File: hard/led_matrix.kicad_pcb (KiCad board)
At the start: 2 copper layers, 150 x 150 mm, 14 parts, among them J1 MicroXNJ

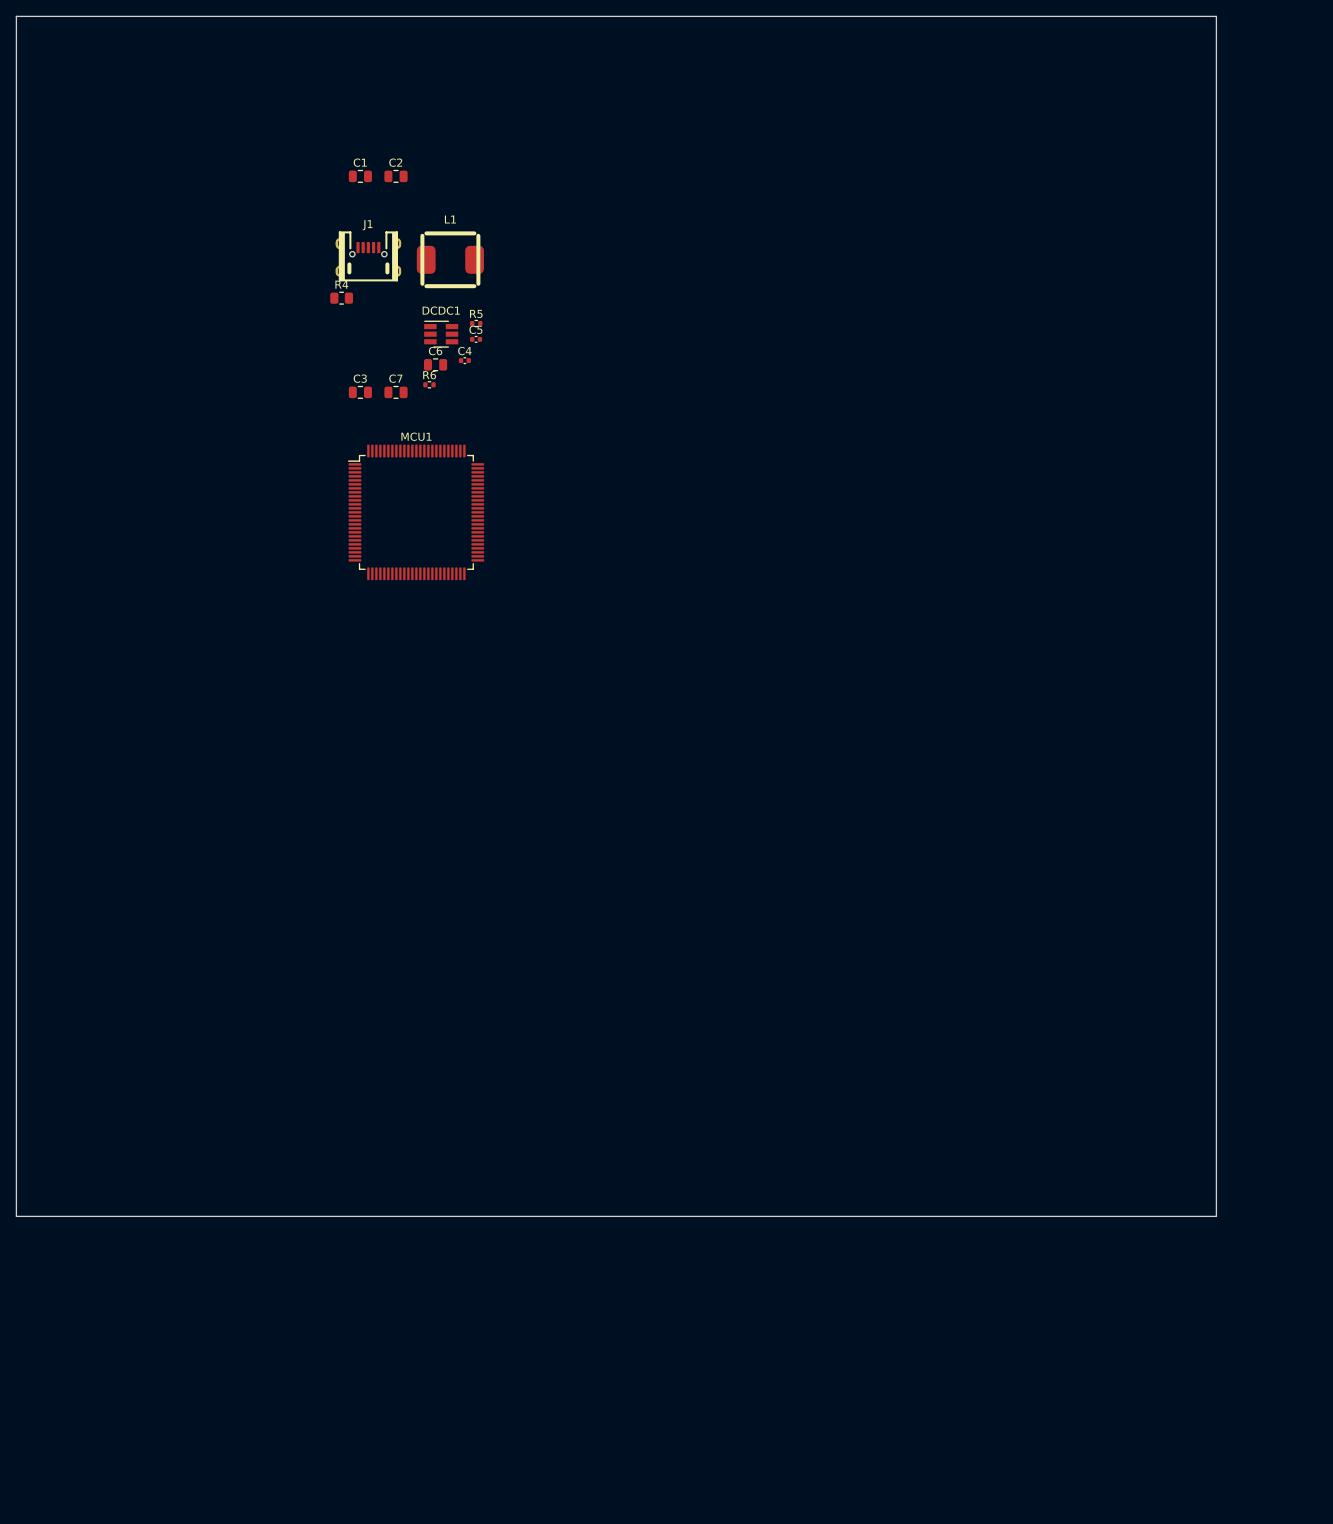
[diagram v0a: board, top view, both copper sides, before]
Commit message: RIIIIIIIIIIIIIBSSSSSS!!!!
Rib break
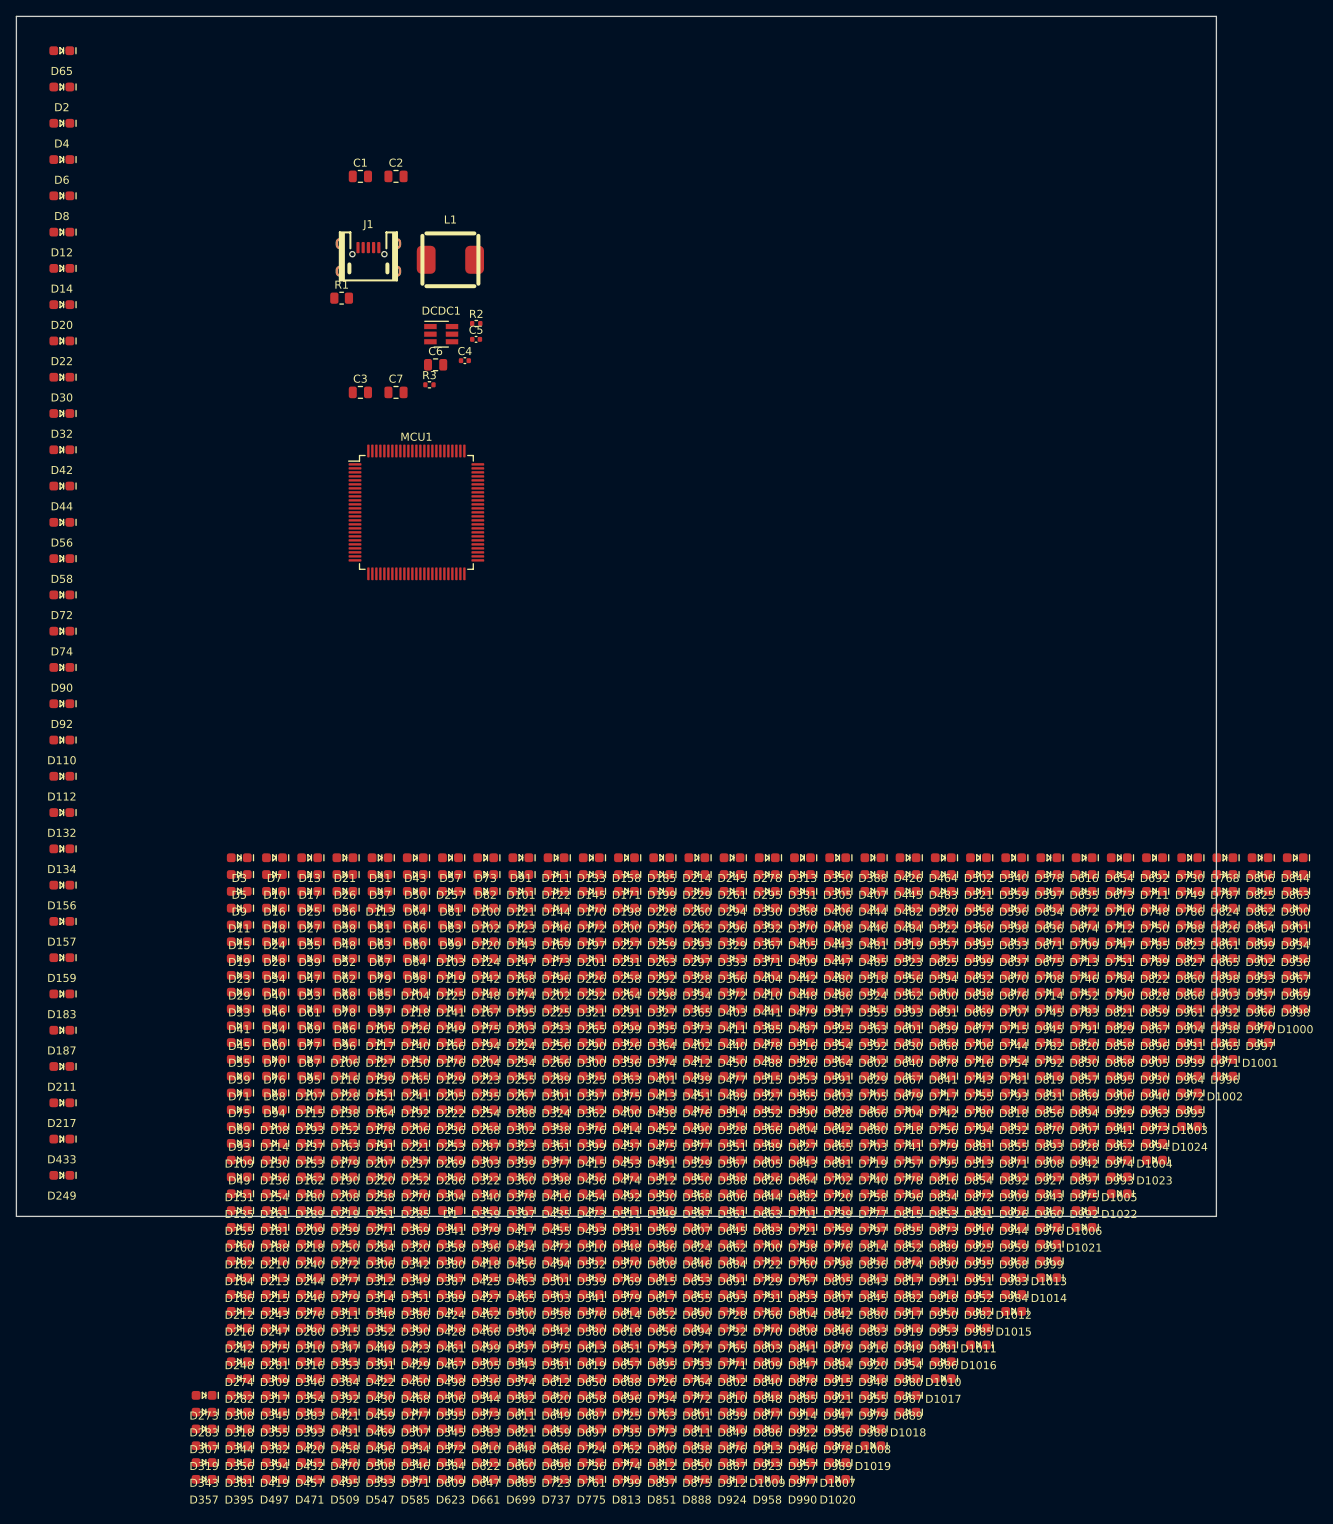
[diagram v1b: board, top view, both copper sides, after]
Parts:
- added D1: LTST-S270TBKT, led_matrix:LED_LiteOn_LTST-S270TBKT, F.Cu at (74.3, 177.2)
- added D10: LTST-S270TBKT, led_matrix:LED_LiteOn_LTST-S270TBKT, F.Cu at (52.3, 137.3)
- added D100: LTST-S270TBKT, led_matrix:LED_LiteOn_LTST-S270TBKT, F.Cu at (78.7, 139.4)
- added D1000: LTST-S270TBKT, led_matrix:LED_LiteOn_LTST-S270TBKT, F.Cu at (179.9, 154.1)
- added D1001: LTST-S270TBKT, led_matrix:LED_LiteOn_LTST-S270TBKT, F.Cu at (175.5, 158.3)
- added D1002: LTST-S270TBKT, led_matrix:LED_LiteOn_LTST-S270TBKT, F.Cu at (171.1, 162.5)
- added D1003: LTST-S270TBKT, led_matrix:LED_LiteOn_LTST-S270TBKT, F.Cu at (166.7, 166.7)
- added D1004: LTST-S270TBKT, led_matrix:LED_LiteOn_LTST-S270TBKT, F.Cu at (162.3, 170.9)
- added D1005: LTST-S270TBKT, led_matrix:LED_LiteOn_LTST-S270TBKT, F.Cu at (157.9, 175.1)
- added D1006: LTST-S270TBKT, led_matrix:LED_LiteOn_LTST-S270TBKT, F.Cu at (153.5, 179.3)
- added D1007: LTST-S270TBKT, led_matrix:LED_LiteOn_LTST-S270TBKT, F.Cu at (122.7, 210.8)
- added D1008: LTST-S270TBKT, led_matrix:LED_LiteOn_LTST-S270TBKT, F.Cu at (127.1, 206.6)
- added D1009: LTST-S270TBKT, led_matrix:LED_LiteOn_LTST-S270TBKT, F.Cu at (113.9, 210.8)
- added D101: LTST-S270TBKT, led_matrix:LED_LiteOn_LTST-S270TBKT, F.Cu at (83.1, 137.3)
- added D1010: LTST-S270TBKT, led_matrix:LED_LiteOn_LTST-S270TBKT, F.Cu at (135.9, 198.2)
- added D1011: LTST-S270TBKT, led_matrix:LED_LiteOn_LTST-S270TBKT, F.Cu at (140.3, 194.0)
- added D1012: LTST-S270TBKT, led_matrix:LED_LiteOn_LTST-S270TBKT, F.Cu at (144.7, 189.8)
- added D1013: LTST-S270TBKT, led_matrix:LED_LiteOn_LTST-S270TBKT, F.Cu at (149.1, 185.6)
- added D1014: LTST-S270TBKT, led_matrix:LED_LiteOn_LTST-S270TBKT, F.Cu at (149.1, 187.7)
- added D1015: LTST-S270TBKT, led_matrix:LED_LiteOn_LTST-S270TBKT, F.Cu at (144.7, 191.9)
- added D1016: LTST-S270TBKT, led_matrix:LED_LiteOn_LTST-S270TBKT, F.Cu at (140.3, 196.1)
- added D1017: LTST-S270TBKT, led_matrix:LED_LiteOn_LTST-S270TBKT, F.Cu at (135.9, 200.3)
- added D1018: LTST-S270TBKT, led_matrix:LED_LiteOn_LTST-S270TBKT, F.Cu at (131.5, 204.5)
- added D1019: LTST-S270TBKT, led_matrix:LED_LiteOn_LTST-S270TBKT, F.Cu at (127.1, 208.7)
- added D102: LTST-S270TBKT, led_matrix:LED_LiteOn_LTST-S270TBKT, F.Cu at (78.7, 141.5)
- added D1020: LTST-S270TBKT, led_matrix:LED_LiteOn_LTST-S270TBKT, F.Cu at (122.7, 212.9)
- added D1021: LTST-S270TBKT, led_matrix:LED_LiteOn_LTST-S270TBKT, F.Cu at (153.5, 181.4)
- added D1022: LTST-S270TBKT, led_matrix:LED_LiteOn_LTST-S270TBKT, F.Cu at (157.9, 177.2)
- added D1023: LTST-S270TBKT, led_matrix:LED_LiteOn_LTST-S270TBKT, F.Cu at (162.3, 173.0)
- added D1024: LTST-S270TBKT, led_matrix:LED_LiteOn_LTST-S270TBKT, F.Cu at (166.7, 168.8)
- added D103: LTST-S270TBKT, led_matrix:LED_LiteOn_LTST-S270TBKT, F.Cu at (74.3, 145.7)
- added D104: LTST-S270TBKT, led_matrix:LED_LiteOn_LTST-S270TBKT, F.Cu at (69.9, 149.9)
- added D105: LTST-S270TBKT, led_matrix:LED_LiteOn_LTST-S270TBKT, F.Cu at (65.5, 154.1)
- added D106: LTST-S270TBKT, led_matrix:LED_LiteOn_LTST-S270TBKT, F.Cu at (61.1, 158.3)
- added D107: LTST-S270TBKT, led_matrix:LED_LiteOn_LTST-S270TBKT, F.Cu at (56.7, 162.5)
- added D108: LTST-S270TBKT, led_matrix:LED_LiteOn_LTST-S270TBKT, F.Cu at (52.3, 166.7)
- added D109: LTST-S270TBKT, led_matrix:LED_LiteOn_LTST-S270TBKT, F.Cu at (47.9, 170.9)
- added D11: LTST-S270TBKT, led_matrix:LED_LiteOn_LTST-S270TBKT, F.Cu at (47.9, 141.5)
- added D110: LTST-S270TBKT, led_matrix:LED_LiteOn_LTST-S270TBKT, F.Cu at (25.7, 120.5)
- added D111: LTST-S270TBKT, led_matrix:LED_LiteOn_LTST-S270TBKT, F.Cu at (87.5, 135.2)
- added D112: LTST-S270TBKT, led_matrix:LED_LiteOn_LTST-S270TBKT, F.Cu at (25.7, 125.0)
- added D113: LTST-S270TBKT, led_matrix:LED_LiteOn_LTST-S270TBKT, F.Cu at (65.5, 139.4)
- added D114: LTST-S270TBKT, led_matrix:LED_LiteOn_LTST-S270TBKT, F.Cu at (52.3, 168.8)
- added D115: LTST-S270TBKT, led_matrix:LED_LiteOn_LTST-S270TBKT, F.Cu at (56.7, 164.6)
- added D116: LTST-S270TBKT, led_matrix:LED_LiteOn_LTST-S270TBKT, F.Cu at (61.1, 160.4)
- added D117: LTST-S270TBKT, led_matrix:LED_LiteOn_LTST-S270TBKT, F.Cu at (65.5, 156.2)
- added D118: LTST-S270TBKT, led_matrix:LED_LiteOn_LTST-S270TBKT, F.Cu at (69.9, 152.0)
- added D119: LTST-S270TBKT, led_matrix:LED_LiteOn_LTST-S270TBKT, F.Cu at (74.3, 147.8)
- added D12: LTST-S270TBKT, led_matrix:LED_LiteOn_LTST-S270TBKT, F.Cu at (25.7, 57.0)
- added D120: LTST-S270TBKT, led_matrix:LED_LiteOn_LTST-S270TBKT, F.Cu at (78.7, 143.6)
- added D121: LTST-S270TBKT, led_matrix:LED_LiteOn_LTST-S270TBKT, F.Cu at (83.1, 139.4)
- added D122: LTST-S270TBKT, led_matrix:LED_LiteOn_LTST-S270TBKT, F.Cu at (87.5, 137.3)
- added D123: LTST-S270TBKT, led_matrix:LED_LiteOn_LTST-S270TBKT, F.Cu at (83.1, 141.5)
- added D124: LTST-S270TBKT, led_matrix:LED_LiteOn_LTST-S270TBKT, F.Cu at (78.7, 145.7)
- added D125: LTST-S270TBKT, led_matrix:LED_LiteOn_LTST-S270TBKT, F.Cu at (74.3, 149.9)
- added D126: LTST-S270TBKT, led_matrix:LED_LiteOn_LTST-S270TBKT, F.Cu at (69.9, 154.1)
- added D127: LTST-S270TBKT, led_matrix:LED_LiteOn_LTST-S270TBKT, F.Cu at (65.5, 158.3)
- added D128: LTST-S270TBKT, led_matrix:LED_LiteOn_LTST-S270TBKT, F.Cu at (61.1, 162.5)
- added D129: LTST-S270TBKT, led_matrix:LED_LiteOn_LTST-S270TBKT, F.Cu at (74.3, 160.4)
- added D13: LTST-S270TBKT, led_matrix:LED_LiteOn_LTST-S270TBKT, F.Cu at (56.7, 135.2)
- added D130: LTST-S270TBKT, led_matrix:LED_LiteOn_LTST-S270TBKT, F.Cu at (52.3, 170.9)
- added D131: LTST-S270TBKT, led_matrix:LED_LiteOn_LTST-S270TBKT, F.Cu at (47.9, 175.1)
- added D132: LTST-S270TBKT, led_matrix:LED_LiteOn_LTST-S270TBKT, F.Cu at (25.7, 129.5)
- added D133: LTST-S270TBKT, led_matrix:LED_LiteOn_LTST-S270TBKT, F.Cu at (91.9, 135.2)
- added D134: LTST-S270TBKT, led_matrix:LED_LiteOn_LTST-S270TBKT, F.Cu at (25.7, 134.1)
- added D135: LTST-S270TBKT, led_matrix:LED_LiteOn_LTST-S270TBKT, F.Cu at (47.9, 177.2)
- added D136: LTST-S270TBKT, led_matrix:LED_LiteOn_LTST-S270TBKT, F.Cu at (52.3, 173.0)
- added D137: LTST-S270TBKT, led_matrix:LED_LiteOn_LTST-S270TBKT, F.Cu at (56.7, 168.8)
- added D138: LTST-S270TBKT, led_matrix:LED_LiteOn_LTST-S270TBKT, F.Cu at (61.1, 164.6)
- added D139: LTST-S270TBKT, led_matrix:LED_LiteOn_LTST-S270TBKT, F.Cu at (65.5, 160.4)
- added D14: LTST-S270TBKT, led_matrix:LED_LiteOn_LTST-S270TBKT, F.Cu at (25.7, 61.5)
- added D140: LTST-S270TBKT, led_matrix:LED_LiteOn_LTST-S270TBKT, F.Cu at (69.9, 156.2)
- added D141: LTST-S270TBKT, led_matrix:LED_LiteOn_LTST-S270TBKT, F.Cu at (74.3, 152.0)
- added D142: LTST-S270TBKT, led_matrix:LED_LiteOn_LTST-S270TBKT, F.Cu at (78.7, 147.8)
- added D143: LTST-S270TBKT, led_matrix:LED_LiteOn_LTST-S270TBKT, F.Cu at (83.1, 143.6)
- added D144: LTST-S270TBKT, led_matrix:LED_LiteOn_LTST-S270TBKT, F.Cu at (87.5, 139.4)
- added D145: LTST-S270TBKT, led_matrix:LED_LiteOn_LTST-S270TBKT, F.Cu at (91.9, 137.3)
- added D146: LTST-S270TBKT, led_matrix:LED_LiteOn_LTST-S270TBKT, F.Cu at (87.5, 141.5)
- added D147: LTST-S270TBKT, led_matrix:LED_LiteOn_LTST-S270TBKT, F.Cu at (83.1, 145.7)
- added D148: LTST-S270TBKT, led_matrix:LED_LiteOn_LTST-S270TBKT, F.Cu at (78.7, 149.9)
- added D149: LTST-S270TBKT, led_matrix:LED_LiteOn_LTST-S270TBKT, F.Cu at (74.3, 154.1)
- added D15: LTST-S270TBKT, led_matrix:LED_LiteOn_LTST-S270TBKT, F.Cu at (47.9, 143.6)
- added D150: LTST-S270TBKT, led_matrix:LED_LiteOn_LTST-S270TBKT, F.Cu at (69.9, 158.3)
- added D151: LTST-S270TBKT, led_matrix:LED_LiteOn_LTST-S270TBKT, F.Cu at (65.5, 162.5)
- added D152: LTST-S270TBKT, led_matrix:LED_LiteOn_LTST-S270TBKT, F.Cu at (61.1, 166.7)
- added D153: LTST-S270TBKT, led_matrix:LED_LiteOn_LTST-S270TBKT, F.Cu at (56.7, 170.9)
- added D154: LTST-S270TBKT, led_matrix:LED_LiteOn_LTST-S270TBKT, F.Cu at (52.3, 175.1)
- added D155: LTST-S270TBKT, led_matrix:LED_LiteOn_LTST-S270TBKT, F.Cu at (47.9, 179.3)
- added D156: LTST-S270TBKT, led_matrix:LED_LiteOn_LTST-S270TBKT, F.Cu at (25.7, 138.6)
- added D157: LTST-S270TBKT, led_matrix:LED_LiteOn_LTST-S270TBKT, F.Cu at (25.7, 143.1)
- added D158: LTST-S270TBKT, led_matrix:LED_LiteOn_LTST-S270TBKT, F.Cu at (96.3, 135.2)
- added D159: LTST-S270TBKT, led_matrix:LED_LiteOn_LTST-S270TBKT, F.Cu at (25.7, 147.7)
- added D16: LTST-S270TBKT, led_matrix:LED_LiteOn_LTST-S270TBKT, F.Cu at (52.3, 139.4)
- added D160: LTST-S270TBKT, led_matrix:LED_LiteOn_LTST-S270TBKT, F.Cu at (47.9, 181.4)
- added D161: LTST-S270TBKT, led_matrix:LED_LiteOn_LTST-S270TBKT, F.Cu at (52.3, 177.2)
- added D162: LTST-S270TBKT, led_matrix:LED_LiteOn_LTST-S270TBKT, F.Cu at (56.7, 173.0)
- added D163: LTST-S270TBKT, led_matrix:LED_LiteOn_LTST-S270TBKT, F.Cu at (61.1, 168.8)
- added D164: LTST-S270TBKT, led_matrix:LED_LiteOn_LTST-S270TBKT, F.Cu at (65.5, 164.6)
- added D165: LTST-S270TBKT, led_matrix:LED_LiteOn_LTST-S270TBKT, F.Cu at (69.9, 160.4)
- added D166: LTST-S270TBKT, led_matrix:LED_LiteOn_LTST-S270TBKT, F.Cu at (74.3, 156.2)
- added D167: LTST-S270TBKT, led_matrix:LED_LiteOn_LTST-S270TBKT, F.Cu at (78.7, 152.0)
- added D168: LTST-S270TBKT, led_matrix:LED_LiteOn_LTST-S270TBKT, F.Cu at (83.1, 147.8)
- added D169: LTST-S270TBKT, led_matrix:LED_LiteOn_LTST-S270TBKT, F.Cu at (87.5, 143.6)
- added D17: LTST-S270TBKT, led_matrix:LED_LiteOn_LTST-S270TBKT, F.Cu at (56.7, 137.3)
- added D170: LTST-S270TBKT, led_matrix:LED_LiteOn_LTST-S270TBKT, F.Cu at (91.9, 139.4)
- added D171: LTST-S270TBKT, led_matrix:LED_LiteOn_LTST-S270TBKT, F.Cu at (96.3, 137.3)
- added D172: LTST-S270TBKT, led_matrix:LED_LiteOn_LTST-S270TBKT, F.Cu at (91.9, 141.5)
- added D173: LTST-S270TBKT, led_matrix:LED_LiteOn_LTST-S270TBKT, F.Cu at (87.5, 145.7)
- added D174: LTST-S270TBKT, led_matrix:LED_LiteOn_LTST-S270TBKT, F.Cu at (83.1, 149.9)
- added D175: LTST-S270TBKT, led_matrix:LED_LiteOn_LTST-S270TBKT, F.Cu at (78.7, 154.1)
- added D176: LTST-S270TBKT, led_matrix:LED_LiteOn_LTST-S270TBKT, F.Cu at (74.3, 158.3)
- added D177: LTST-S270TBKT, led_matrix:LED_LiteOn_LTST-S270TBKT, F.Cu at (69.9, 202.4)
- added D178: LTST-S270TBKT, led_matrix:LED_LiteOn_LTST-S270TBKT, F.Cu at (65.5, 166.7)
- added D179: LTST-S270TBKT, led_matrix:LED_LiteOn_LTST-S270TBKT, F.Cu at (61.1, 170.9)
- added D18: LTST-S270TBKT, led_matrix:LED_LiteOn_LTST-S270TBKT, F.Cu at (52.3, 141.5)
- added D180: LTST-S270TBKT, led_matrix:LED_LiteOn_LTST-S270TBKT, F.Cu at (56.7, 175.1)
- added D181: LTST-S270TBKT, led_matrix:LED_LiteOn_LTST-S270TBKT, F.Cu at (52.3, 179.3)
- added D182: LTST-S270TBKT, led_matrix:LED_LiteOn_LTST-S270TBKT, F.Cu at (47.9, 183.5)
- added D183: LTST-S270TBKT, led_matrix:LED_LiteOn_LTST-S270TBKT, F.Cu at (25.7, 152.2)
- added D184: LTST-S270TBKT, led_matrix:LED_LiteOn_LTST-S270TBKT, F.Cu at (47.9, 185.6)
- added D185: LTST-S270TBKT, led_matrix:LED_LiteOn_LTST-S270TBKT, F.Cu at (100.7, 135.2)
- added D186: LTST-S270TBKT, led_matrix:LED_LiteOn_LTST-S270TBKT, F.Cu at (47.9, 187.7)
- added D187: LTST-S270TBKT, led_matrix:LED_LiteOn_LTST-S270TBKT, F.Cu at (25.7, 156.7)
- added D188: LTST-S270TBKT, led_matrix:LED_LiteOn_LTST-S270TBKT, F.Cu at (52.3, 181.4)
- added D189: LTST-S270TBKT, led_matrix:LED_LiteOn_LTST-S270TBKT, F.Cu at (56.7, 177.2)
- added D19: LTST-S270TBKT, led_matrix:LED_LiteOn_LTST-S270TBKT, F.Cu at (47.9, 145.7)
- added D190: LTST-S270TBKT, led_matrix:LED_LiteOn_LTST-S270TBKT, F.Cu at (61.1, 173.0)
- added D191: LTST-S270TBKT, led_matrix:LED_LiteOn_LTST-S270TBKT, F.Cu at (65.5, 168.8)
- added D192: LTST-S270TBKT, led_matrix:LED_LiteOn_LTST-S270TBKT, F.Cu at (69.9, 164.6)
- added D193: LTST-S270TBKT, led_matrix:LED_LiteOn_LTST-S270TBKT, F.Cu at (56.7, 166.7)
- added D194: LTST-S270TBKT, led_matrix:LED_LiteOn_LTST-S270TBKT, F.Cu at (78.7, 156.2)
- added D195: LTST-S270TBKT, led_matrix:LED_LiteOn_LTST-S270TBKT, F.Cu at (83.1, 152.0)
- added D196: LTST-S270TBKT, led_matrix:LED_LiteOn_LTST-S270TBKT, F.Cu at (87.5, 147.8)
- added D197: LTST-S270TBKT, led_matrix:LED_LiteOn_LTST-S270TBKT, F.Cu at (91.9, 143.6)
- added D198: LTST-S270TBKT, led_matrix:LED_LiteOn_LTST-S270TBKT, F.Cu at (96.3, 139.4)
- added D199: LTST-S270TBKT, led_matrix:LED_LiteOn_LTST-S270TBKT, F.Cu at (100.7, 137.3)
- added D2: LTST-S270TBKT, led_matrix:LED_LiteOn_LTST-S270TBKT, F.Cu at (25.7, 38.8)
- added D20: LTST-S270TBKT, led_matrix:LED_LiteOn_LTST-S270TBKT, F.Cu at (25.7, 66.0)
- added D200: LTST-S270TBKT, led_matrix:LED_LiteOn_LTST-S270TBKT, F.Cu at (96.3, 141.5)
- added D201: LTST-S270TBKT, led_matrix:LED_LiteOn_LTST-S270TBKT, F.Cu at (91.9, 145.7)
- added D202: LTST-S270TBKT, led_matrix:LED_LiteOn_LTST-S270TBKT, F.Cu at (87.5, 149.9)
- added D203: LTST-S270TBKT, led_matrix:LED_LiteOn_LTST-S270TBKT, F.Cu at (83.1, 154.1)
- added D204: LTST-S270TBKT, led_matrix:LED_LiteOn_LTST-S270TBKT, F.Cu at (78.7, 158.3)
- added D205: LTST-S270TBKT, led_matrix:LED_LiteOn_LTST-S270TBKT, F.Cu at (74.3, 162.5)
- added D206: LTST-S270TBKT, led_matrix:LED_LiteOn_LTST-S270TBKT, F.Cu at (69.9, 166.7)
- added D207: LTST-S270TBKT, led_matrix:LED_LiteOn_LTST-S270TBKT, F.Cu at (65.5, 170.9)
- added D208: LTST-S270TBKT, led_matrix:LED_LiteOn_LTST-S270TBKT, F.Cu at (61.1, 175.1)
- added D209: LTST-S270TBKT, led_matrix:LED_LiteOn_LTST-S270TBKT, F.Cu at (56.7, 179.3)
- added D21: LTST-S270TBKT, led_matrix:LED_LiteOn_LTST-S270TBKT, F.Cu at (61.1, 135.2)
- added D210: LTST-S270TBKT, led_matrix:LED_LiteOn_LTST-S270TBKT, F.Cu at (52.3, 183.5)
- added D211: LTST-S270TBKT, led_matrix:LED_LiteOn_LTST-S270TBKT, F.Cu at (25.7, 161.3)
- added D212: LTST-S270TBKT, led_matrix:LED_LiteOn_LTST-S270TBKT, F.Cu at (47.9, 189.8)
- added D213: LTST-S270TBKT, led_matrix:LED_LiteOn_LTST-S270TBKT, F.Cu at (52.3, 185.6)
- added D214: LTST-S270TBKT, led_matrix:LED_LiteOn_LTST-S270TBKT, F.Cu at (105.1, 135.2)
- added D215: LTST-S270TBKT, led_matrix:LED_LiteOn_LTST-S270TBKT, F.Cu at (52.3, 187.7)
- added D216: LTST-S270TBKT, led_matrix:LED_LiteOn_LTST-S270TBKT, F.Cu at (47.9, 191.9)
- added D217: LTST-S270TBKT, led_matrix:LED_LiteOn_LTST-S270TBKT, F.Cu at (25.7, 165.8)
- added D218: LTST-S270TBKT, led_matrix:LED_LiteOn_LTST-S270TBKT, F.Cu at (56.7, 181.4)
- added D219: LTST-S270TBKT, led_matrix:LED_LiteOn_LTST-S270TBKT, F.Cu at (61.1, 177.2)
- added D22: LTST-S270TBKT, led_matrix:LED_LiteOn_LTST-S270TBKT, F.Cu at (25.7, 70.6)
- added D220: LTST-S270TBKT, led_matrix:LED_LiteOn_LTST-S270TBKT, F.Cu at (65.5, 173.0)
- added D221: LTST-S270TBKT, led_matrix:LED_LiteOn_LTST-S270TBKT, F.Cu at (69.9, 168.8)
- added D222: LTST-S270TBKT, led_matrix:LED_LiteOn_LTST-S270TBKT, F.Cu at (74.3, 164.6)
- added D223: LTST-S270TBKT, led_matrix:LED_LiteOn_LTST-S270TBKT, F.Cu at (78.7, 160.4)
- added D224: LTST-S270TBKT, led_matrix:LED_LiteOn_LTST-S270TBKT, F.Cu at (83.1, 156.2)
- added D225: LTST-S270TBKT, led_matrix:LED_LiteOn_LTST-S270TBKT, F.Cu at (87.5, 152.0)
- added D226: LTST-S270TBKT, led_matrix:LED_LiteOn_LTST-S270TBKT, F.Cu at (91.9, 147.8)
- added D227: LTST-S270TBKT, led_matrix:LED_LiteOn_LTST-S270TBKT, F.Cu at (96.3, 143.6)
- added D228: LTST-S270TBKT, led_matrix:LED_LiteOn_LTST-S270TBKT, F.Cu at (100.7, 139.4)
- added D229: LTST-S270TBKT, led_matrix:LED_LiteOn_LTST-S270TBKT, F.Cu at (105.1, 137.3)
- added D23: LTST-S270TBKT, led_matrix:LED_LiteOn_LTST-S270TBKT, F.Cu at (47.9, 147.8)
- added D230: LTST-S270TBKT, led_matrix:LED_LiteOn_LTST-S270TBKT, F.Cu at (100.7, 141.5)
- added D231: LTST-S270TBKT, led_matrix:LED_LiteOn_LTST-S270TBKT, F.Cu at (96.3, 145.7)
- added D232: LTST-S270TBKT, led_matrix:LED_LiteOn_LTST-S270TBKT, F.Cu at (91.9, 149.9)
- added D233: LTST-S270TBKT, led_matrix:LED_LiteOn_LTST-S270TBKT, F.Cu at (87.5, 154.1)
- added D234: LTST-S270TBKT, led_matrix:LED_LiteOn_LTST-S270TBKT, F.Cu at (83.1, 158.3)
- added D235: LTST-S270TBKT, led_matrix:LED_LiteOn_LTST-S270TBKT, F.Cu at (78.7, 162.5)
- added D236: LTST-S270TBKT, led_matrix:LED_LiteOn_LTST-S270TBKT, F.Cu at (74.3, 166.7)
- added D237: LTST-S270TBKT, led_matrix:LED_LiteOn_LTST-S270TBKT, F.Cu at (69.9, 170.9)
- added D238: LTST-S270TBKT, led_matrix:LED_LiteOn_LTST-S270TBKT, F.Cu at (65.5, 175.1)
- added D239: LTST-S270TBKT, led_matrix:LED_LiteOn_LTST-S270TBKT, F.Cu at (61.1, 179.3)
- added D24: LTST-S270TBKT, led_matrix:LED_LiteOn_LTST-S270TBKT, F.Cu at (52.3, 143.6)
- added D240: LTST-S270TBKT, led_matrix:LED_LiteOn_LTST-S270TBKT, F.Cu at (56.7, 183.5)
- added D241: LTST-S270TBKT, led_matrix:LED_LiteOn_LTST-S270TBKT, F.Cu at (69.9, 162.5)
- added D242: LTST-S270TBKT, led_matrix:LED_LiteOn_LTST-S270TBKT, F.Cu at (47.9, 194.0)
- added D243: LTST-S270TBKT, led_matrix:LED_LiteOn_LTST-S270TBKT, F.Cu at (52.3, 189.8)
- added D244: LTST-S270TBKT, led_matrix:LED_LiteOn_LTST-S270TBKT, F.Cu at (56.7, 185.6)
- added D245: LTST-S270TBKT, led_matrix:LED_LiteOn_LTST-S270TBKT, F.Cu at (109.5, 135.2)
- added D246: LTST-S270TBKT, led_matrix:LED_LiteOn_LTST-S270TBKT, F.Cu at (56.7, 187.7)
- added D247: LTST-S270TBKT, led_matrix:LED_LiteOn_LTST-S270TBKT, F.Cu at (52.3, 191.9)
- added D248: LTST-S270TBKT, led_matrix:LED_LiteOn_LTST-S270TBKT, F.Cu at (47.9, 196.1)
- added D249: LTST-S270TBKT, led_matrix:LED_LiteOn_LTST-S270TBKT, F.Cu at (25.7, 174.9)
- added D25: LTST-S270TBKT, led_matrix:LED_LiteOn_LTST-S270TBKT, F.Cu at (56.7, 139.4)
- added D250: LTST-S270TBKT, led_matrix:LED_LiteOn_LTST-S270TBKT, F.Cu at (61.1, 181.4)
- added D251: LTST-S270TBKT, led_matrix:LED_LiteOn_LTST-S270TBKT, F.Cu at (65.5, 177.2)
- added D252: LTST-S270TBKT, led_matrix:LED_LiteOn_LTST-S270TBKT, F.Cu at (69.9, 173.0)
- added D253: LTST-S270TBKT, led_matrix:LED_LiteOn_LTST-S270TBKT, F.Cu at (74.3, 168.8)
- added D254: LTST-S270TBKT, led_matrix:LED_LiteOn_LTST-S270TBKT, F.Cu at (78.7, 164.6)
- added D255: LTST-S270TBKT, led_matrix:LED_LiteOn_LTST-S270TBKT, F.Cu at (83.1, 160.4)
- added D256: LTST-S270TBKT, led_matrix:LED_LiteOn_LTST-S270TBKT, F.Cu at (87.5, 156.2)
- added D257: LTST-S270TBKT, led_matrix:LED_LiteOn_LTST-S270TBKT, F.Cu at (74.3, 137.3)
- added D258: LTST-S270TBKT, led_matrix:LED_LiteOn_LTST-S270TBKT, F.Cu at (96.3, 147.8)
- added D259: LTST-S270TBKT, led_matrix:LED_LiteOn_LTST-S270TBKT, F.Cu at (100.7, 143.6)
- added D26: LTST-S270TBKT, led_matrix:LED_LiteOn_LTST-S270TBKT, F.Cu at (61.1, 137.3)
- added D260: LTST-S270TBKT, led_matrix:LED_LiteOn_LTST-S270TBKT, F.Cu at (105.1, 139.4)
- added D261: LTST-S270TBKT, led_matrix:LED_LiteOn_LTST-S270TBKT, F.Cu at (109.5, 137.3)
- added D262: LTST-S270TBKT, led_matrix:LED_LiteOn_LTST-S270TBKT, F.Cu at (105.1, 141.5)
- added D263: LTST-S270TBKT, led_matrix:LED_LiteOn_LTST-S270TBKT, F.Cu at (100.7, 145.7)
- added D264: LTST-S270TBKT, led_matrix:LED_LiteOn_LTST-S270TBKT, F.Cu at (96.3, 149.9)
- added D265: LTST-S270TBKT, led_matrix:LED_LiteOn_LTST-S270TBKT, F.Cu at (91.9, 154.1)
- added D266: LTST-S270TBKT, led_matrix:LED_LiteOn_LTST-S270TBKT, F.Cu at (87.5, 158.3)
- added D267: LTST-S270TBKT, led_matrix:LED_LiteOn_LTST-S270TBKT, F.Cu at (83.1, 162.5)
- added D268: LTST-S270TBKT, led_matrix:LED_LiteOn_LTST-S270TBKT, F.Cu at (78.7, 166.7)
- added D269: LTST-S270TBKT, led_matrix:LED_LiteOn_LTST-S270TBKT, F.Cu at (74.3, 170.9)
- added D27: LTST-S270TBKT, led_matrix:LED_LiteOn_LTST-S270TBKT, F.Cu at (56.7, 141.5)
- added D270: LTST-S270TBKT, led_matrix:LED_LiteOn_LTST-S270TBKT, F.Cu at (69.9, 175.1)
- added D271: LTST-S270TBKT, led_matrix:LED_LiteOn_LTST-S270TBKT, F.Cu at (65.5, 179.3)
- added D272: LTST-S270TBKT, led_matrix:LED_LiteOn_LTST-S270TBKT, F.Cu at (61.1, 183.5)
- added D273: LTST-S270TBKT, led_matrix:LED_LiteOn_LTST-S270TBKT, F.Cu at (43.5, 202.4)
- added D274: LTST-S270TBKT, led_matrix:LED_LiteOn_LTST-S270TBKT, F.Cu at (47.9, 198.2)
- added D275: LTST-S270TBKT, led_matrix:LED_LiteOn_LTST-S270TBKT, F.Cu at (52.3, 194.0)
- added D276: LTST-S270TBKT, led_matrix:LED_LiteOn_LTST-S270TBKT, F.Cu at (56.7, 189.8)
- added D277: LTST-S270TBKT, led_matrix:LED_LiteOn_LTST-S270TBKT, F.Cu at (61.1, 185.6)
- added D278: LTST-S270TBKT, led_matrix:LED_LiteOn_LTST-S270TBKT, F.Cu at (113.9, 135.2)
- added D279: LTST-S270TBKT, led_matrix:LED_LiteOn_LTST-S270TBKT, F.Cu at (61.1, 187.7)
- added D28: LTST-S270TBKT, led_matrix:LED_LiteOn_LTST-S270TBKT, F.Cu at (52.3, 145.7)
- added D280: LTST-S270TBKT, led_matrix:LED_LiteOn_LTST-S270TBKT, F.Cu at (56.7, 191.9)
- added D281: LTST-S270TBKT, led_matrix:LED_LiteOn_LTST-S270TBKT, F.Cu at (52.3, 196.1)
- added D282: LTST-S270TBKT, led_matrix:LED_LiteOn_LTST-S270TBKT, F.Cu at (47.9, 200.3)
- added D283: LTST-S270TBKT, led_matrix:LED_LiteOn_LTST-S270TBKT, F.Cu at (43.5, 204.5)
- added D284: LTST-S270TBKT, led_matrix:LED_LiteOn_LTST-S270TBKT, F.Cu at (65.5, 181.4)
- added D285: LTST-S270TBKT, led_matrix:LED_LiteOn_LTST-S270TBKT, F.Cu at (69.9, 177.2)
- added D286: LTST-S270TBKT, led_matrix:LED_LiteOn_LTST-S270TBKT, F.Cu at (74.3, 173.0)
- added D287: LTST-S270TBKT, led_matrix:LED_LiteOn_LTST-S270TBKT, F.Cu at (78.7, 168.8)
- added D288: LTST-S270TBKT, led_matrix:LED_LiteOn_LTST-S270TBKT, F.Cu at (83.1, 164.6)
- added D289: LTST-S270TBKT, led_matrix:LED_LiteOn_LTST-S270TBKT, F.Cu at (87.5, 160.4)
- added D29: LTST-S270TBKT, led_matrix:LED_LiteOn_LTST-S270TBKT, F.Cu at (47.9, 149.9)
- added D290: LTST-S270TBKT, led_matrix:LED_LiteOn_LTST-S270TBKT, F.Cu at (91.9, 156.2)
- added D291: LTST-S270TBKT, led_matrix:LED_LiteOn_LTST-S270TBKT, F.Cu at (96.3, 152.0)
- added D292: LTST-S270TBKT, led_matrix:LED_LiteOn_LTST-S270TBKT, F.Cu at (100.7, 147.8)
- added D293: LTST-S270TBKT, led_matrix:LED_LiteOn_LTST-S270TBKT, F.Cu at (105.1, 143.6)
- added D294: LTST-S270TBKT, led_matrix:LED_LiteOn_LTST-S270TBKT, F.Cu at (109.5, 139.4)
- added D295: LTST-S270TBKT, led_matrix:LED_LiteOn_LTST-S270TBKT, F.Cu at (113.9, 137.3)
- added D296: LTST-S270TBKT, led_matrix:LED_LiteOn_LTST-S270TBKT, F.Cu at (109.5, 141.5)
- added D297: LTST-S270TBKT, led_matrix:LED_LiteOn_LTST-S270TBKT, F.Cu at (105.1, 145.7)
- added D298: LTST-S270TBKT, led_matrix:LED_LiteOn_LTST-S270TBKT, F.Cu at (100.7, 149.9)
- added D299: LTST-S270TBKT, led_matrix:LED_LiteOn_LTST-S270TBKT, F.Cu at (96.3, 154.1)
- added D3: LTST-S270TBKT, led_matrix:LED_LiteOn_LTST-S270TBKT, F.Cu at (47.9, 135.2)
- added D30: LTST-S270TBKT, led_matrix:LED_LiteOn_LTST-S270TBKT, F.Cu at (25.7, 75.1)
- added D300: LTST-S270TBKT, led_matrix:LED_LiteOn_LTST-S270TBKT, F.Cu at (91.9, 158.3)
- added D301: LTST-S270TBKT, led_matrix:LED_LiteOn_LTST-S270TBKT, F.Cu at (87.5, 162.5)
- added D302: LTST-S270TBKT, led_matrix:LED_LiteOn_LTST-S270TBKT, F.Cu at (83.1, 166.7)
- added D303: LTST-S270TBKT, led_matrix:LED_LiteOn_LTST-S270TBKT, F.Cu at (78.7, 170.9)
- added D304: LTST-S270TBKT, led_matrix:LED_LiteOn_LTST-S270TBKT, F.Cu at (74.3, 175.1)
- added D305: LTST-S270TBKT, led_matrix:LED_LiteOn_LTST-S270TBKT, F.Cu at (122.7, 137.3)
- added D306: LTST-S270TBKT, led_matrix:LED_LiteOn_LTST-S270TBKT, F.Cu at (65.5, 183.5)
- added D307: LTST-S270TBKT, led_matrix:LED_LiteOn_LTST-S270TBKT, F.Cu at (43.5, 206.6)
- added D308: LTST-S270TBKT, led_matrix:LED_LiteOn_LTST-S270TBKT, F.Cu at (47.9, 202.4)
- added D309: LTST-S270TBKT, led_matrix:LED_LiteOn_LTST-S270TBKT, F.Cu at (52.3, 198.2)
- added D31: LTST-S270TBKT, led_matrix:LED_LiteOn_LTST-S270TBKT, F.Cu at (65.5, 135.2)
- added D310: LTST-S270TBKT, led_matrix:LED_LiteOn_LTST-S270TBKT, F.Cu at (56.7, 194.0)
- added D311: LTST-S270TBKT, led_matrix:LED_LiteOn_LTST-S270TBKT, F.Cu at (61.1, 189.8)
- added D312: LTST-S270TBKT, led_matrix:LED_LiteOn_LTST-S270TBKT, F.Cu at (65.5, 185.6)
- added D313: LTST-S270TBKT, led_matrix:LED_LiteOn_LTST-S270TBKT, F.Cu at (118.3, 135.2)
- added D314: LTST-S270TBKT, led_matrix:LED_LiteOn_LTST-S270TBKT, F.Cu at (65.5, 187.7)
- added D315: LTST-S270TBKT, led_matrix:LED_LiteOn_LTST-S270TBKT, F.Cu at (61.1, 191.9)
- added D316: LTST-S270TBKT, led_matrix:LED_LiteOn_LTST-S270TBKT, F.Cu at (56.7, 196.1)
- added D317: LTST-S270TBKT, led_matrix:LED_LiteOn_LTST-S270TBKT, F.Cu at (52.3, 200.3)
- added D318: LTST-S270TBKT, led_matrix:LED_LiteOn_LTST-S270TBKT, F.Cu at (47.9, 204.5)
- added D319: LTST-S270TBKT, led_matrix:LED_LiteOn_LTST-S270TBKT, F.Cu at (43.5, 208.7)
- added D32: LTST-S270TBKT, led_matrix:LED_LiteOn_LTST-S270TBKT, F.Cu at (25.7, 79.6)
- added D320: LTST-S270TBKT, led_matrix:LED_LiteOn_LTST-S270TBKT, F.Cu at (69.9, 181.4)
- added D321: LTST-S270TBKT, led_matrix:LED_LiteOn_LTST-S270TBKT, F.Cu at (91.9, 152.0)
- added D322: LTST-S270TBKT, led_matrix:LED_LiteOn_LTST-S270TBKT, F.Cu at (78.7, 173.0)
- added D323: LTST-S270TBKT, led_matrix:LED_LiteOn_LTST-S270TBKT, F.Cu at (83.1, 168.8)
- added D324: LTST-S270TBKT, led_matrix:LED_LiteOn_LTST-S270TBKT, F.Cu at (87.5, 164.6)
- added D325: LTST-S270TBKT, led_matrix:LED_LiteOn_LTST-S270TBKT, F.Cu at (91.9, 160.4)
- added D326: LTST-S270TBKT, led_matrix:LED_LiteOn_LTST-S270TBKT, F.Cu at (96.3, 156.2)
- added D327: LTST-S270TBKT, led_matrix:LED_LiteOn_LTST-S270TBKT, F.Cu at (100.7, 152.0)
- added D328: LTST-S270TBKT, led_matrix:LED_LiteOn_LTST-S270TBKT, F.Cu at (105.1, 147.8)
- added D329: LTST-S270TBKT, led_matrix:LED_LiteOn_LTST-S270TBKT, F.Cu at (109.5, 143.6)
- added D33: LTST-S270TBKT, led_matrix:LED_LiteOn_LTST-S270TBKT, F.Cu at (47.9, 152.0)
- added D330: LTST-S270TBKT, led_matrix:LED_LiteOn_LTST-S270TBKT, F.Cu at (113.9, 139.4)
- added D331: LTST-S270TBKT, led_matrix:LED_LiteOn_LTST-S270TBKT, F.Cu at (118.3, 137.3)
- added D332: LTST-S270TBKT, led_matrix:LED_LiteOn_LTST-S270TBKT, F.Cu at (113.9, 141.5)
- added D333: LTST-S270TBKT, led_matrix:LED_LiteOn_LTST-S270TBKT, F.Cu at (109.5, 145.7)
- added D334: LTST-S270TBKT, led_matrix:LED_LiteOn_LTST-S270TBKT, F.Cu at (105.1, 149.9)
- added D335: LTST-S270TBKT, led_matrix:LED_LiteOn_LTST-S270TBKT, F.Cu at (100.7, 154.1)
- added D336: LTST-S270TBKT, led_matrix:LED_LiteOn_LTST-S270TBKT, F.Cu at (96.3, 158.3)
- added D337: LTST-S270TBKT, led_matrix:LED_LiteOn_LTST-S270TBKT, F.Cu at (91.9, 162.5)
- added D338: LTST-S270TBKT, led_matrix:LED_LiteOn_LTST-S270TBKT, F.Cu at (87.5, 166.7)
- added D339: LTST-S270TBKT, led_matrix:LED_LiteOn_LTST-S270TBKT, F.Cu at (83.1, 170.9)
- added D34: LTST-S270TBKT, led_matrix:LED_LiteOn_LTST-S270TBKT, F.Cu at (52.3, 147.8)
- added D340: LTST-S270TBKT, led_matrix:LED_LiteOn_LTST-S270TBKT, F.Cu at (78.7, 175.1)
- added D341: LTST-S270TBKT, led_matrix:LED_LiteOn_LTST-S270TBKT, F.Cu at (74.3, 179.3)
- added D342: LTST-S270TBKT, led_matrix:LED_LiteOn_LTST-S270TBKT, F.Cu at (69.9, 183.5)
- added D343: LTST-S270TBKT, led_matrix:LED_LiteOn_LTST-S270TBKT, F.Cu at (43.5, 210.8)
- added D344: LTST-S270TBKT, led_matrix:LED_LiteOn_LTST-S270TBKT, F.Cu at (47.9, 206.6)
- added D345: LTST-S270TBKT, led_matrix:LED_LiteOn_LTST-S270TBKT, F.Cu at (52.3, 202.4)
- added D346: LTST-S270TBKT, led_matrix:LED_LiteOn_LTST-S270TBKT, F.Cu at (56.7, 198.2)
- added D347: LTST-S270TBKT, led_matrix:LED_LiteOn_LTST-S270TBKT, F.Cu at (61.1, 194.0)
- added D348: LTST-S270TBKT, led_matrix:LED_LiteOn_LTST-S270TBKT, F.Cu at (65.5, 189.8)
- added D349: LTST-S270TBKT, led_matrix:LED_LiteOn_LTST-S270TBKT, F.Cu at (69.9, 185.6)
- added D35: LTST-S270TBKT, led_matrix:LED_LiteOn_LTST-S270TBKT, F.Cu at (56.7, 143.6)
- added D350: LTST-S270TBKT, led_matrix:LED_LiteOn_LTST-S270TBKT, F.Cu at (122.7, 135.2)
- added D351: LTST-S270TBKT, led_matrix:LED_LiteOn_LTST-S270TBKT, F.Cu at (69.9, 187.7)
- added D352: LTST-S270TBKT, led_matrix:LED_LiteOn_LTST-S270TBKT, F.Cu at (65.5, 191.9)
- added D353: LTST-S270TBKT, led_matrix:LED_LiteOn_LTST-S270TBKT, F.Cu at (61.1, 196.1)
- added D354: LTST-S270TBKT, led_matrix:LED_LiteOn_LTST-S270TBKT, F.Cu at (56.7, 200.3)
- added D355: LTST-S270TBKT, led_matrix:LED_LiteOn_LTST-S270TBKT, F.Cu at (52.3, 204.5)
- added D356: LTST-S270TBKT, led_matrix:LED_LiteOn_LTST-S270TBKT, F.Cu at (47.9, 208.7)
- added D357: LTST-S270TBKT, led_matrix:LED_LiteOn_LTST-S270TBKT, F.Cu at (43.5, 212.9)
- added D358: LTST-S270TBKT, led_matrix:LED_LiteOn_LTST-S270TBKT, F.Cu at (74.3, 181.4)
- added D359: LTST-S270TBKT, led_matrix:LED_LiteOn_LTST-S270TBKT, F.Cu at (78.7, 177.2)
- added D36: LTST-S270TBKT, led_matrix:LED_LiteOn_LTST-S270TBKT, F.Cu at (61.1, 139.4)
- added D360: LTST-S270TBKT, led_matrix:LED_LiteOn_LTST-S270TBKT, F.Cu at (83.1, 173.0)
- added D361: LTST-S270TBKT, led_matrix:LED_LiteOn_LTST-S270TBKT, F.Cu at (87.5, 168.8)
- added D362: LTST-S270TBKT, led_matrix:LED_LiteOn_LTST-S270TBKT, F.Cu at (91.9, 164.6)
- added D363: LTST-S270TBKT, led_matrix:LED_LiteOn_LTST-S270TBKT, F.Cu at (96.3, 160.4)
- added D364: LTST-S270TBKT, led_matrix:LED_LiteOn_LTST-S270TBKT, F.Cu at (100.7, 156.2)
- added D365: LTST-S270TBKT, led_matrix:LED_LiteOn_LTST-S270TBKT, F.Cu at (105.1, 152.0)
- added D366: LTST-S270TBKT, led_matrix:LED_LiteOn_LTST-S270TBKT, F.Cu at (109.5, 147.8)
- added D367: LTST-S270TBKT, led_matrix:LED_LiteOn_LTST-S270TBKT, F.Cu at (113.9, 143.6)
- added D368: LTST-S270TBKT, led_matrix:LED_LiteOn_LTST-S270TBKT, F.Cu at (118.3, 139.4)
- added D369: LTST-S270TBKT, led_matrix:LED_LiteOn_LTST-S270TBKT, F.Cu at (69.9, 179.3)
- added D37: LTST-S270TBKT, led_matrix:LED_LiteOn_LTST-S270TBKT, F.Cu at (65.5, 137.3)
- added D370: LTST-S270TBKT, led_matrix:LED_LiteOn_LTST-S270TBKT, F.Cu at (118.3, 141.5)
- added D371: LTST-S270TBKT, led_matrix:LED_LiteOn_LTST-S270TBKT, F.Cu at (113.9, 145.7)
- added D372: LTST-S270TBKT, led_matrix:LED_LiteOn_LTST-S270TBKT, F.Cu at (109.5, 149.9)
- added D373: LTST-S270TBKT, led_matrix:LED_LiteOn_LTST-S270TBKT, F.Cu at (105.1, 154.1)
- added D374: LTST-S270TBKT, led_matrix:LED_LiteOn_LTST-S270TBKT, F.Cu at (100.7, 158.3)
- added D375: LTST-S270TBKT, led_matrix:LED_LiteOn_LTST-S270TBKT, F.Cu at (96.3, 162.5)
- added D376: LTST-S270TBKT, led_matrix:LED_LiteOn_LTST-S270TBKT, F.Cu at (91.9, 166.7)
- added D377: LTST-S270TBKT, led_matrix:LED_LiteOn_LTST-S270TBKT, F.Cu at (87.5, 170.9)
- added D378: LTST-S270TBKT, led_matrix:LED_LiteOn_LTST-S270TBKT, F.Cu at (83.1, 175.1)
- added D379: LTST-S270TBKT, led_matrix:LED_LiteOn_LTST-S270TBKT, F.Cu at (78.7, 179.3)
- added D38: LTST-S270TBKT, led_matrix:LED_LiteOn_LTST-S270TBKT, F.Cu at (61.1, 141.5)
- added D380: LTST-S270TBKT, led_matrix:LED_LiteOn_LTST-S270TBKT, F.Cu at (74.3, 183.5)
- added D381: LTST-S270TBKT, led_matrix:LED_LiteOn_LTST-S270TBKT, F.Cu at (47.9, 210.8)
- added D382: LTST-S270TBKT, led_matrix:LED_LiteOn_LTST-S270TBKT, F.Cu at (52.3, 206.6)
- added D383: LTST-S270TBKT, led_matrix:LED_LiteOn_LTST-S270TBKT, F.Cu at (56.7, 202.4)
- added D384: LTST-S270TBKT, led_matrix:LED_LiteOn_LTST-S270TBKT, F.Cu at (61.1, 198.2)
- added D385: LTST-S270TBKT, led_matrix:LED_LiteOn_LTST-S270TBKT, F.Cu at (113.9, 154.1)
- added D386: LTST-S270TBKT, led_matrix:LED_LiteOn_LTST-S270TBKT, F.Cu at (69.9, 189.8)
- added D387: LTST-S270TBKT, led_matrix:LED_LiteOn_LTST-S270TBKT, F.Cu at (74.3, 185.6)
- added D388: LTST-S270TBKT, led_matrix:LED_LiteOn_LTST-S270TBKT, F.Cu at (127.1, 135.2)
- added D389: LTST-S270TBKT, led_matrix:LED_LiteOn_LTST-S270TBKT, F.Cu at (74.3, 187.7)
- added D39: LTST-S270TBKT, led_matrix:LED_LiteOn_LTST-S270TBKT, F.Cu at (56.7, 145.7)
- renumbered R4 to R1, R5 to R2, R6 to R3
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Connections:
- DCDC1 pad 5: (no net) -> Net-(DCDC1-Pad5)
- J1 pad 2: (no net) -> Net-(J1-Pad2)
- J1 pad 3: (no net) -> Net-(J1-Pad3)
- J1 pad 4: (no net) -> Net-(J1-Pad4)
- MCU1 pad 1: (no net) -> Net-(MCU1-Pad1)
- MCU1 pad 10: (no net) -> Net-(MCU1-Pad10)
- MCU1 pad 100: (no net) -> Net-(MCU1-Pad100)
- MCU1 pad 11: (no net) -> Net-(MCU1-Pad11)
- MCU1 pad 12: (no net) -> Net-(MCU1-Pad12)
- MCU1 pad 13: (no net) -> Net-(MCU1-Pad13)
- MCU1 pad 14: (no net) -> Net-(MCU1-Pad14)
- MCU1 pad 15: (no net) -> Net-(MCU1-Pad15)
- MCU1 pad 16: (no net) -> Net-(MCU1-Pad16)
- MCU1 pad 17: (no net) -> Net-(MCU1-Pad17)
- MCU1 pad 18: (no net) -> Net-(MCU1-Pad18)
- MCU1 pad 19: (no net) -> Net-(MCU1-Pad19)
- MCU1 pad 2: (no net) -> Net-(MCU1-Pad2)
- MCU1 pad 20: (no net) -> Net-(MCU1-Pad20)
- MCU1 pad 21: (no net) -> Net-(MCU1-Pad21)
- MCU1 pad 22: (no net) -> Net-(MCU1-Pad22)
- MCU1 pad 23: (no net) -> Net-(MCU1-Pad23)
- MCU1 pad 24: (no net) -> Net-(MCU1-Pad24)
- MCU1 pad 25: (no net) -> Net-(MCU1-Pad25)
- MCU1 pad 26: (no net) -> Net-(MCU1-Pad26)
- MCU1 pad 27: (no net) -> Net-(MCU1-Pad27)
- MCU1 pad 28: (no net) -> Net-(MCU1-Pad28)
- MCU1 pad 29: (no net) -> Net-(MCU1-Pad29)
- MCU1 pad 3: (no net) -> Net-(MCU1-Pad3)
- MCU1 pad 30: (no net) -> Net-(MCU1-Pad30)
- MCU1 pad 31: (no net) -> Net-(MCU1-Pad31)
- MCU1 pad 32: (no net) -> Net-(MCU1-Pad32)
- MCU1 pad 33: (no net) -> Net-(MCU1-Pad33)
- MCU1 pad 34: (no net) -> Net-(MCU1-Pad34)
- MCU1 pad 35: (no net) -> Net-(MCU1-Pad35)
- MCU1 pad 36: (no net) -> Net-(MCU1-Pad36)
- MCU1 pad 37: (no net) -> Net-(MCU1-Pad37)
- MCU1 pad 38: (no net) -> Net-(MCU1-Pad38)
- MCU1 pad 39: (no net) -> Net-(MCU1-Pad39)
- MCU1 pad 4: (no net) -> Net-(MCU1-Pad4)
- MCU1 pad 40: (no net) -> Net-(MCU1-Pad40)
- MCU1 pad 41: (no net) -> Net-(MCU1-Pad41)
- MCU1 pad 42: (no net) -> Net-(MCU1-Pad42)
- MCU1 pad 43: (no net) -> Net-(MCU1-Pad43)
- MCU1 pad 44: (no net) -> Net-(MCU1-Pad44)
- MCU1 pad 45: (no net) -> Net-(MCU1-Pad45)
- MCU1 pad 46: (no net) -> Net-(MCU1-Pad46)
- MCU1 pad 47: (no net) -> Net-(MCU1-Pad47)
- MCU1 pad 48: (no net) -> Net-(MCU1-Pad48)
- MCU1 pad 49: (no net) -> Net-(MCU1-Pad49)
- MCU1 pad 5: (no net) -> Net-(MCU1-Pad5)
- MCU1 pad 50: (no net) -> Net-(MCU1-Pad50)
- MCU1 pad 51: (no net) -> Net-(MCU1-Pad51)
- MCU1 pad 52: (no net) -> Net-(MCU1-Pad52)
- MCU1 pad 53: (no net) -> Net-(MCU1-Pad53)
- MCU1 pad 54: (no net) -> Net-(MCU1-Pad54)
- MCU1 pad 55: (no net) -> Net-(MCU1-Pad55)
- MCU1 pad 56: (no net) -> Net-(MCU1-Pad56)
- MCU1 pad 57: (no net) -> Net-(MCU1-Pad57)
- MCU1 pad 58: (no net) -> Net-(MCU1-Pad58)
- MCU1 pad 59: (no net) -> Net-(MCU1-Pad59)
- MCU1 pad 6: (no net) -> Net-(MCU1-Pad6)
- MCU1 pad 60: (no net) -> Net-(MCU1-Pad60)
- MCU1 pad 61: (no net) -> Net-(MCU1-Pad61)
- MCU1 pad 62: (no net) -> Net-(MCU1-Pad62)
- MCU1 pad 63: (no net) -> Net-(MCU1-Pad63)
- MCU1 pad 64: (no net) -> Net-(MCU1-Pad64)
- MCU1 pad 65: (no net) -> Net-(MCU1-Pad65)
- MCU1 pad 66: (no net) -> Net-(MCU1-Pad66)
- MCU1 pad 67: (no net) -> Net-(MCU1-Pad67)
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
